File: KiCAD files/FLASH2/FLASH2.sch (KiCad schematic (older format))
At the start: 15 parts, among them J1 card addr, J2 Power Bus, J3 Signal Bus, J4 IDE connector, U1 74LS04, U2 74LS85, U3 74LS245, U4 74LS245

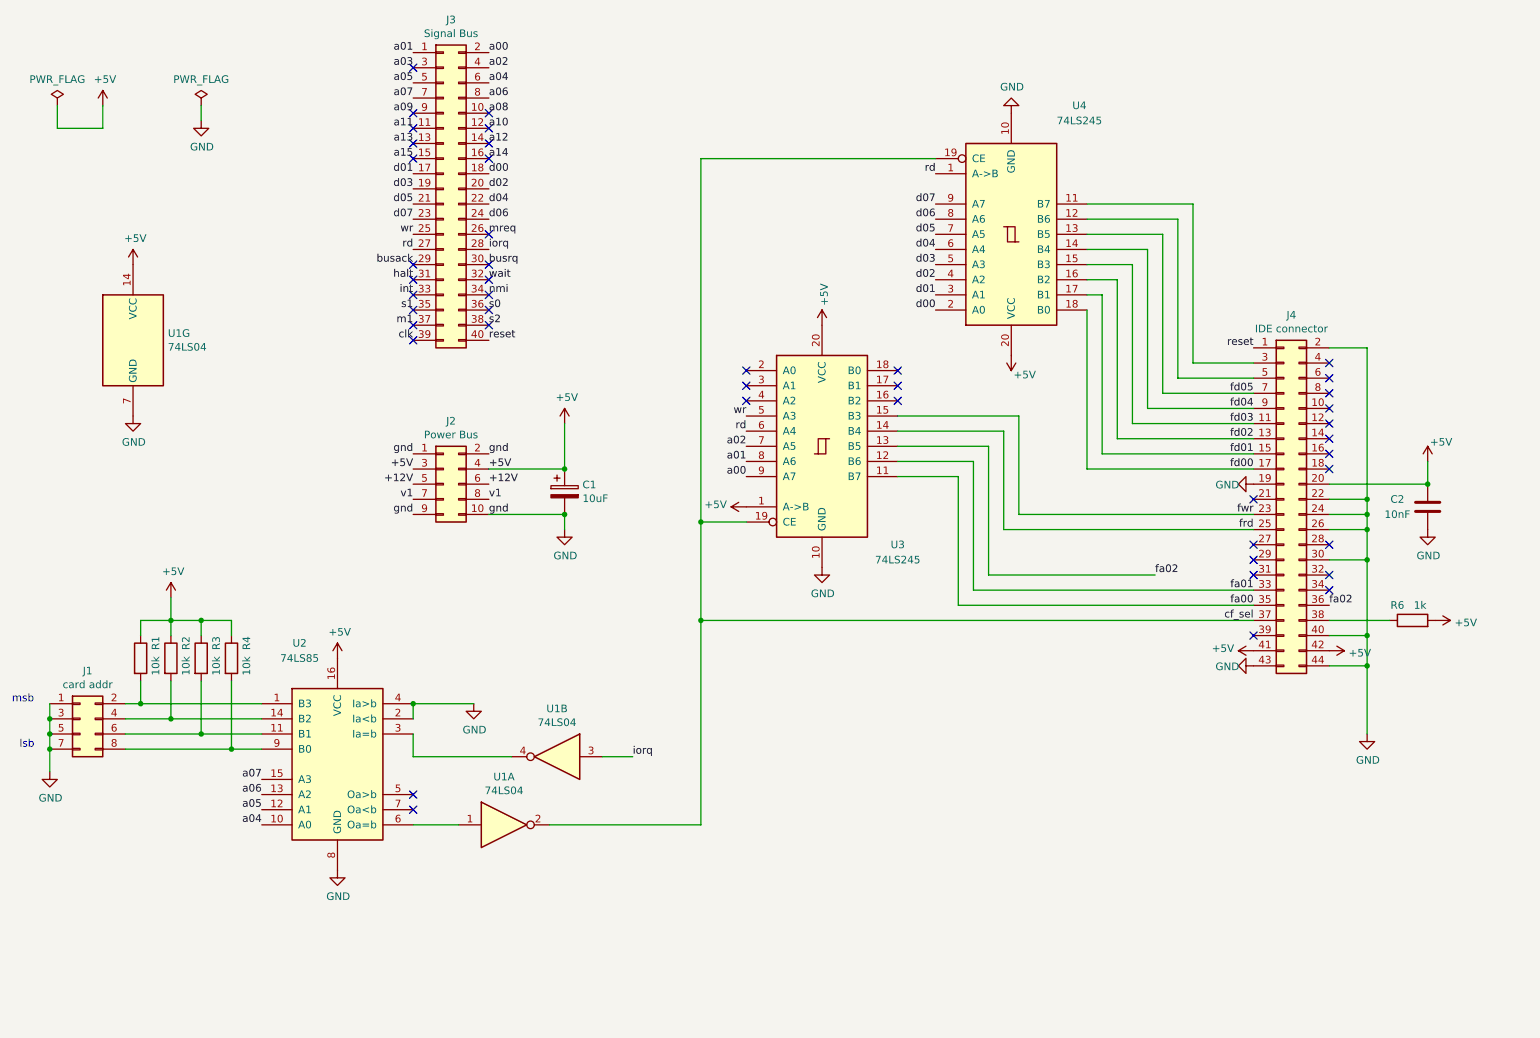
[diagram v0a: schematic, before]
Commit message: Update FLASH2.sch
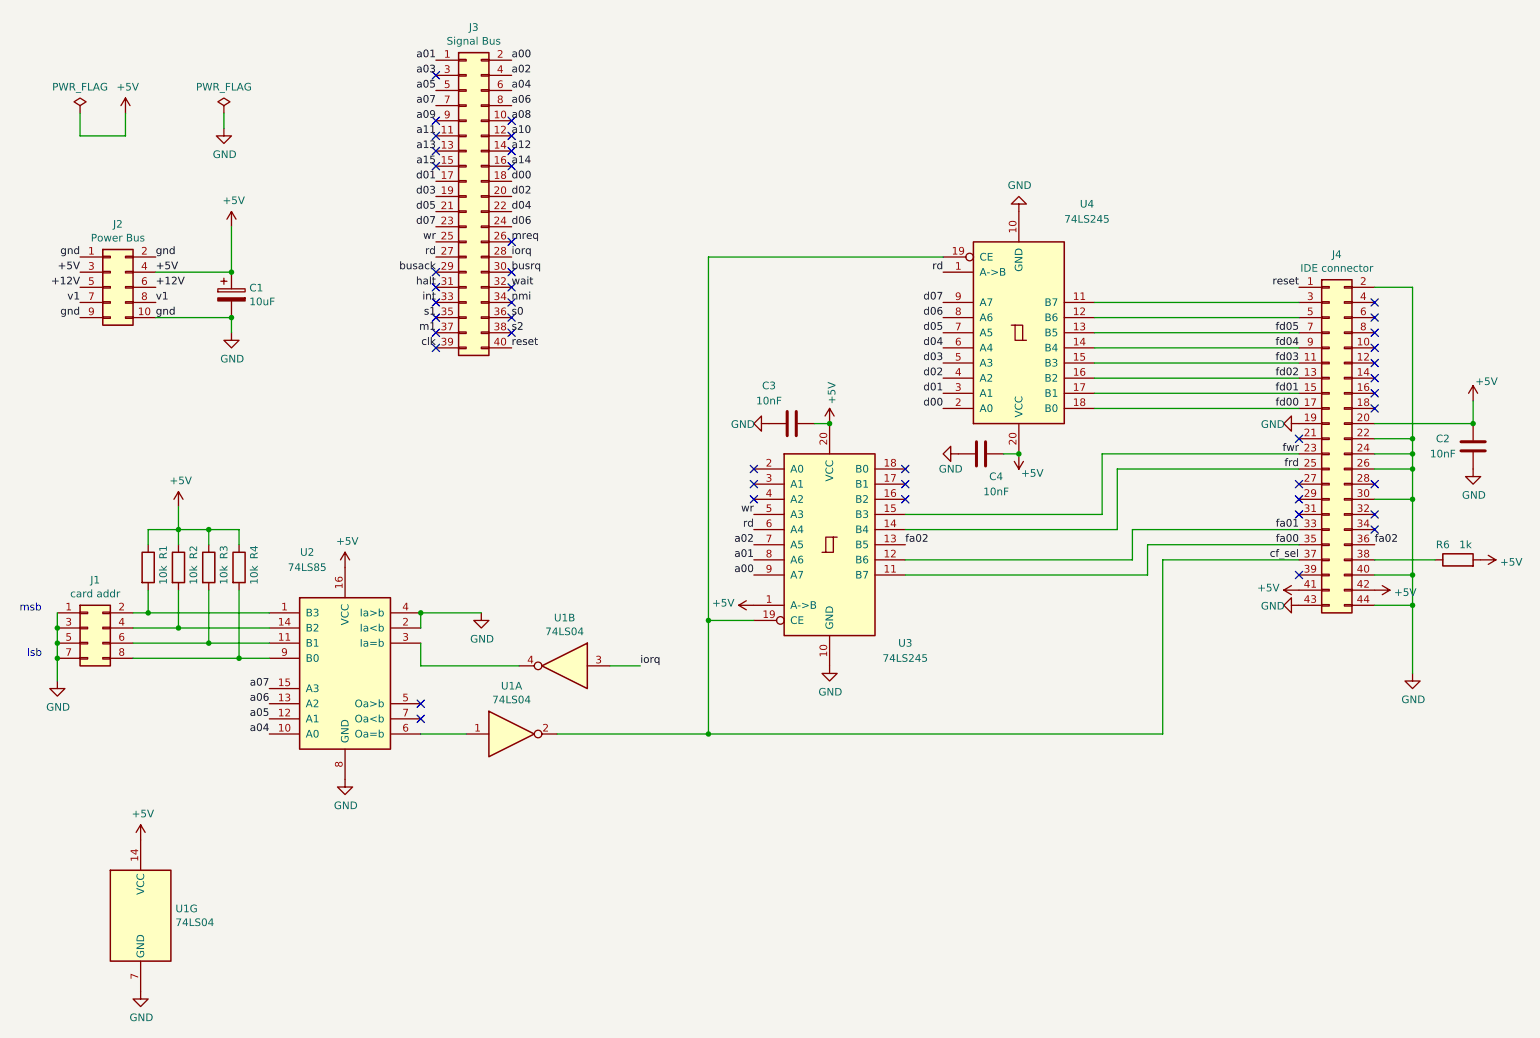
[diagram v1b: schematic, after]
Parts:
- added C3, C4: 10nF, symbol Device:C
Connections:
- net +5V: now also C3.1, C4.1
- net GND: now also C3.2, C4.2
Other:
- moved on the sheet: C1, C2, J1, J2, J3, J4, R1, R2, R3, R4, R6, U1A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
